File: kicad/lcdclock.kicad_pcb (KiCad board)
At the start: 2 copper layers, 102 x 102 mm, 25 parts, among them CON1 AVR-ISP, SW1 RESET, U1 ATTINY24A, U2 AY0438, U3 AY0438, U4 LCD_DE377, U5 CONRAD_DCF, Y1 32.768kHz/12.5pF

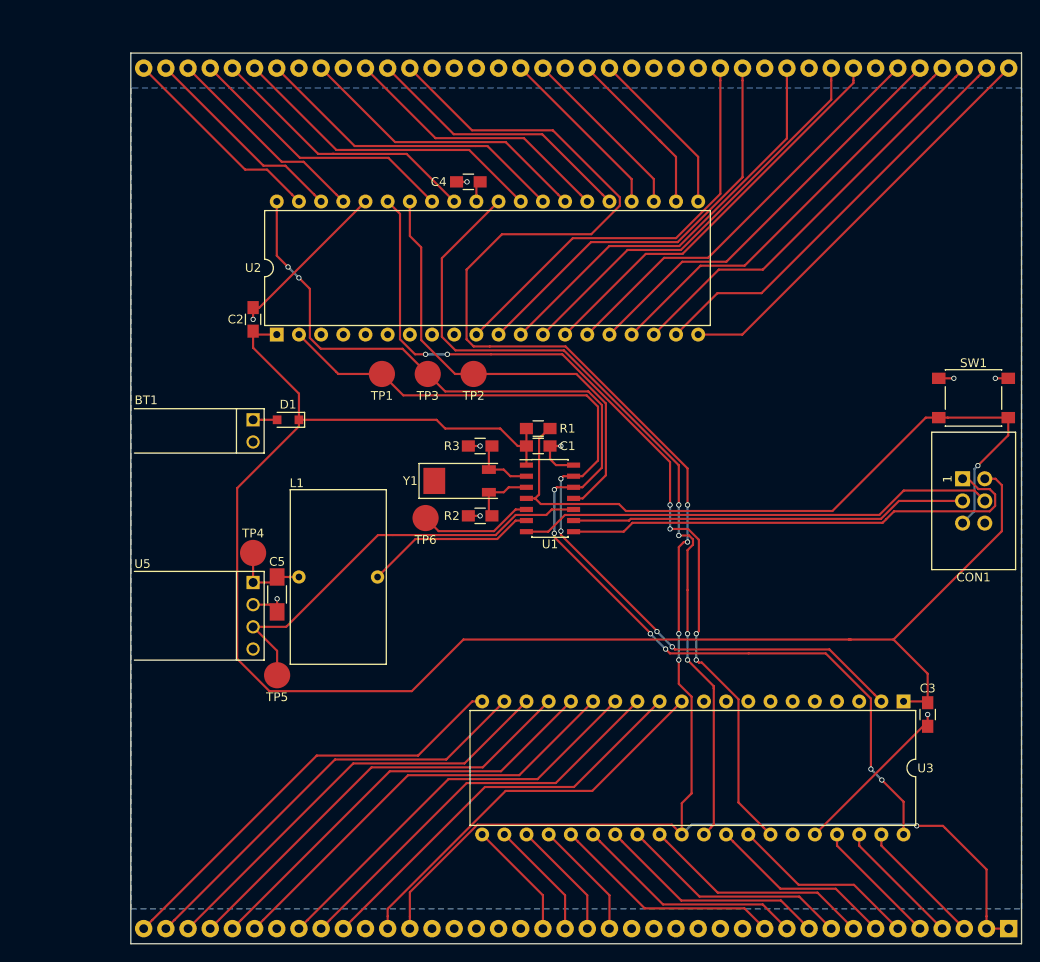
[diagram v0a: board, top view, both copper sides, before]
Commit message: Place components on PCB
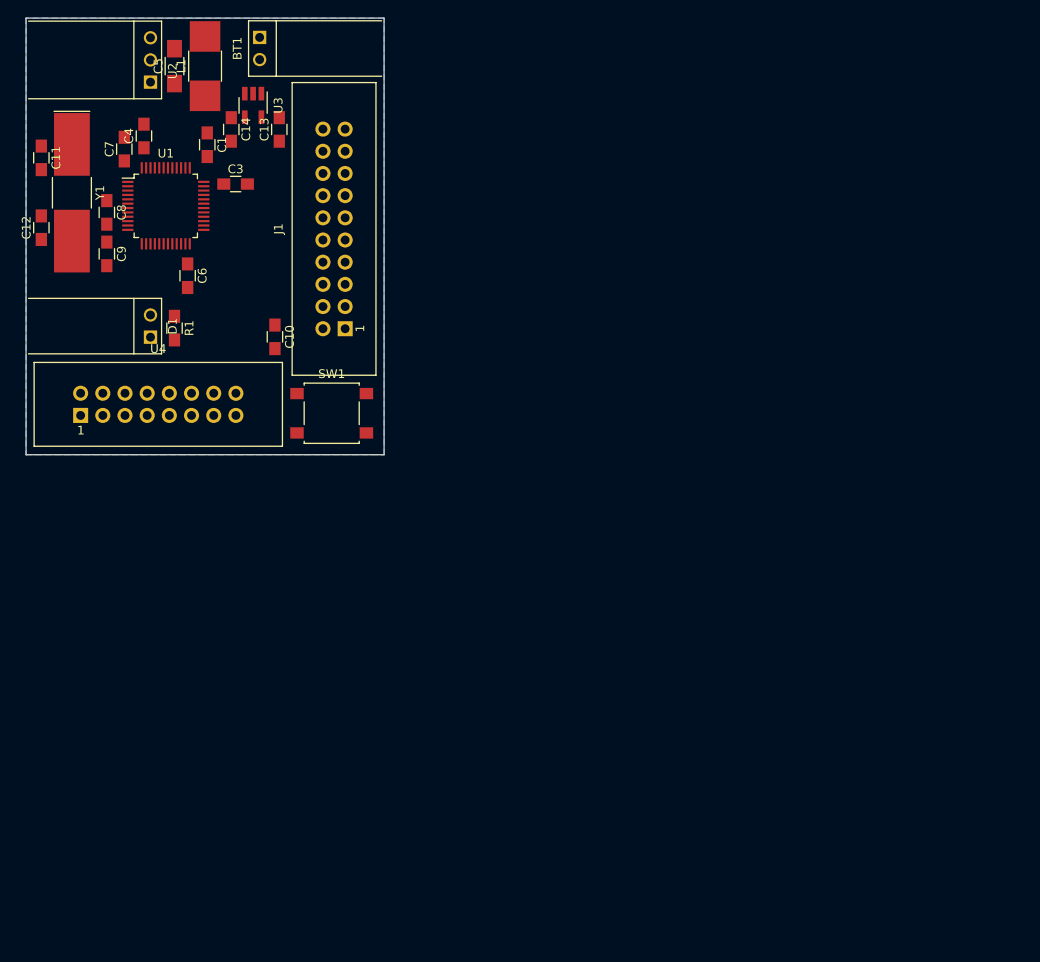
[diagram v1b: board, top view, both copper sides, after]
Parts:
- removed C2: 100n, Resistors_SMD:R_0805_HandSoldering
- removed CON1: AVR-ISP, Connectors:IDC_Header_Straight_6pins
- removed R2, R3: 0, Resistors_SMD:R_0805_HandSoldering
- removed TP1: DLOA, Measurement_Points:Measurement_Point_Round-SMD-Pad_Big
- removed TP2: DDAT, Measurement_Points:Measurement_Point_Round-SMD-Pad_Big
- removed TP3: DCLK, Measurement_Points:Measurement_Point_Round-SMD-Pad_Big
- removed TP4: TVCC, Measurement_Points:Measurement_Point_Round-SMD-Pad_Big
- removed TP5: TSIG, Measurement_Points:Measurement_Point_Round-SMD-Pad_Big
- removed TP6: CLK, Measurement_Points:Measurement_Point_Round-SMD-Pad_Big
- removed U5: CONRAD_DCF, LCD Clock:CONNECTOR_4x1
- added C10: 100n, Resistors_SMD:R_0805_HandSoldering, F.Cu at (48.5, 56.5)
- added C11: 15p, Resistors_SMD:R_0805_HandSoldering, F.Cu at (21.8, 36.0)
- added C12: 15p, Resistors_SMD:R_0805_HandSoldering, F.Cu at (21.8, 44.0)
- added C13: 2.2u, Resistors_SMD:R_0805_HandSoldering, F.Cu at (49.0, 32.8)
- added C14: 1u, Resistors_SMD:R_0805_HandSoldering, F.Cu at (43.5, 32.8)
- added C6: 100n, Resistors_SMD:R_0805_HandSoldering, F.Cu at (38.5, 49.5)
- added C7: 100n, Resistors_SMD:R_0805_HandSoldering, F.Cu at (31.2, 35.0)
- added C8: 100n, Resistors_SMD:R_0805_HandSoldering, F.Cu at (29.2, 42.2)
- added C9: 1u, Resistors_SMD:R_0805_HandSoldering, F.Cu at (29.2, 47.0)
- added J1: Conn_JLink_SWD, Connectors:IDC_Header_Straight_20pins, F.Cu at (56.5, 55.6)
- BT1: value 3.6V Lithium AA -> 4xAA 6.4-3.2V
- C1: value 100n -> 10u
- C4: value 120p -> 100n
- D1: value BAT60A -> LED; footprint Diodes_SMD:D_SOD-323_HandSoldering -> LCD Clock:CONNECTOR_2x1
- L1: footprint LCD Clock:WE_470uH_Inductor -> Resistors_SMD:R_1812_HandSoldering
- R1: value 10k -> 100k
- SW1: value RESET -> SW_Push; footprint Buttons_Switches_SMD:SW_SPST_PTS645 -> Buttons_Switches_SMD:SW_SPST_B3S-1000
- U1: value ATTINY24A -> STM32L073xx_48; footprint Housings_SOIC:SOIC-14_3.9x8.7mm_Pitch1.27mm -> Housings_QFP:LQFP-48_7x7mm_Pitch0.5mm
- U2: value AY0438 -> ELV_DCF-2; footprint Housings_DIP:DIP-40_W15.24mm -> LCD Clock:CONNECTOR_3x1
- U3: value AY0438 -> TPS70630; footprint Housings_DIP:DIP-40_W15.24mm -> TO_SOT_Packages_SMD:SOT-23-5_HandSoldering
- U4: value LCD_DE377 -> LCD; footprint LCD Clock:LCD-DIP -> Connectors:IDC_Header_Straight_16pins; moved to F.Cu
- Y1: value 32.768kHz/12.5pF -> 32.768kHz 12.5pF; footprint LCD Clock:MS1V-T1K -> Crystals:Crystal_SMD_SeikoEpson_MC405-2pin_9.6x4.1mm_HandSoldering
- moved U3 101.0 mm to (46.0, 30.0)
- moved C3 99.9 mm to (44.0, 39.0), turned to 0 degrees
- moved SW1 73.5 mm to (55.0, 65.2)
- moved L1 61.7 mm to (40.5, 25.5), turned to 90 degrees
- moved C5 61.6 mm to (37.0, 25.5)
- moved U4 57.5 mm to (26.2, 65.5), turned to 0 degrees
- moved U1 55.3 mm to (36.0, 41.5)
- moved Y1 54.0 mm to (25.2, 40.0), turned to 270 degrees
- moved C1 51.3 mm to (40.8, 34.5), turned to 270 degrees
- moved BT1 46.3 mm to (46.8, 22.2), turned to 270 degrees
- moved R1 43.2 mm to (37.0, 55.5), turned to 270 degrees
- moved C4 37.5 mm to (33.5, 33.5), turned to 90 degrees
- moved U2 32.3 mm to (34.2, 27.3)
- moved D1 18.4 mm to (34.2, 56.5), turned to 90 degrees
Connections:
- C1 pad 1: +BATT -> VCC
- C3 pad 1: +BATT -> VCC
- C4 pad 1: Net-(C4-Pad1) -> VCC
- D1 pad 1: +BATT -> GND
- D1 pad 2: Net-(BT1-Pad1) -> Net-(D1-Pad2)
- R1 pad 1: +BATT -> Net-(D1-Pad2)
- R1 pad 2: Net-(CON1-Pad5) -> Net-(R1-Pad2)
- SW1 pad 2: Net-(CON1-Pad5) -> Net-(C10-Pad2)
- U1 pad 1: +BATT -> VCC
- U1 pad 10: Net-(TP5-Pad1) -> (no net)
- U1 pad 11: Net-(TP2-Pad1) -> Net-(U1-Pad11)
- U1 pad 12: Net-(TP3-Pad1) -> Net-(U1-Pad12)
- U1 pad 13: Net-(TP1-Pad1) -> Net-(U1-Pad13)
- U1 pad 14: GND -> Net-(L1-Pad1)
- U1 pad 2: Net-(R3-Pad2) -> (no net)
- U1 pad 3: Net-(R2-Pad2) -> Net-(C11-Pad1)
- U1 pad 4: Net-(CON1-Pad5) -> Net-(C12-Pad1)
- U1 pad 5: Net-(TP6-Pad1) -> (no net)
- U1 pad 6: Net-(L1-Pad1) -> (no net)
- U1 pad 7: Net-(CON1-Pad4) -> Net-(C10-Pad2)
- U1 pad 8: Net-(CON1-Pad1) -> GND
- U1 pad 9: Net-(CON1-Pad3) -> VCC
- U2 pad 1: +BATT -> Net-(C5-Pad2)
- U2 pad 2: Net-(TP1-Pad1) -> Net-(U1-Pad15)
- U2 pad 3: (no net) -> GND
- U3 pad 1: +BATT -> Net-(BT1-Pad1)
- U3 pad 2: Net-(TP1-Pad1) -> GND
- U3 pad 3: (no net) -> Net-(BT1-Pad1)
- U3 pad 5: (no net) -> VCC
- U4 pad 1: Net-(U3-Pad30) -> Net-(U1-Pad11)
- U4 pad 10: Net-(U3-Pad27) -> Net-(U1-Pad41)
- U4 pad 11: Net-(U3-Pad26) -> Net-(U1-Pad21)
- U4 pad 12: Net-(U3-Pad25) -> Net-(U1-Pad22)
- U4 pad 13: (no net) -> Net-(U1-Pad46)
- U4 pad 14: (no net) -> Net-(U1-Pad31)
- U4 pad 15: (no net) -> Net-(U1-Pad30)
- U4 pad 16: (no net) -> Net-(U1-Pad29)
- U4 pad 2: Net-(U3-Pad30) -> Net-(U1-Pad12)
- U4 pad 3: Net-(U3-Pad39) -> Net-(U1-Pad13)
- U4 pad 4: Net-(U3-Pad38) -> Net-(U1-Pad16)
- U4 pad 5: Net-(U3-Pad37) -> Net-(U1-Pad17)
- U4 pad 6: Net-(U3-Pad33) -> Net-(U1-Pad18)
- U4 pad 7: Net-(U3-Pad32) -> Net-(U1-Pad19)
- U4 pad 8: Net-(U3-Pad29) -> Net-(U1-Pad39)
- U4 pad 9: Net-(U3-Pad28) -> Net-(U1-Pad40)
- Y1 pad 1: Net-(R3-Pad2) -> Net-(C11-Pad1)
- Y1 pad 2: Net-(R2-Pad2) -> Net-(C12-Pad1)
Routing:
- net Net-(U3-Pad30): track 220.6 -> 0.00 mm, vias 5 -> 0
- net +BATT: track 193.1 -> 0.00 mm
- net Net-(TP3-Pad1): track 134.0 -> 0.00 mm, vias 8 -> 0
- net Net-(U2-Pad35): track 102.2 -> 0.00 mm, vias 6 -> 0
- net Net-(TP1-Pad1): track 100.0 -> 0.00 mm, vias 4 -> 0
- net Net-(U2-Pad30): track 97.1 -> 0.00 mm, vias 4 -> 0
- net Net-(CON1-Pad5): track 83.7 -> 0.00 mm, vias 1 -> 0
- net GND: track 56.2 -> 0.00 mm, vias 9 -> 0
- net Net-(CON1-Pad1): track 55.3 -> 0.00 mm
- net Net-(CON1-Pad4): track 54.9 -> 0.00 mm
- net Net-(TP2-Pad1): track 53.6 -> 0.00 mm
- net Net-(U3-Pad20): track 49.5 -> 0.00 mm
- net Net-(U3-Pad18): track 49.5 -> 0.00 mm
- net Net-(U3-Pad19): track 49.5 -> 0.00 mm
- net Net-(U3-Pad15): track 49.5 -> 0.00 mm
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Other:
- board size 102 x 102 mm -> 41 x 50 mm
